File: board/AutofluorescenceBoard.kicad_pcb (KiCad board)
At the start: 2 copper layers, 57.2 x 45.7 mm, 41 parts, among them J1 2002411212, Q1 BSS138, U1 PAM2863ECR, U2 PAM2863ECR, U3 PAM2863ECR

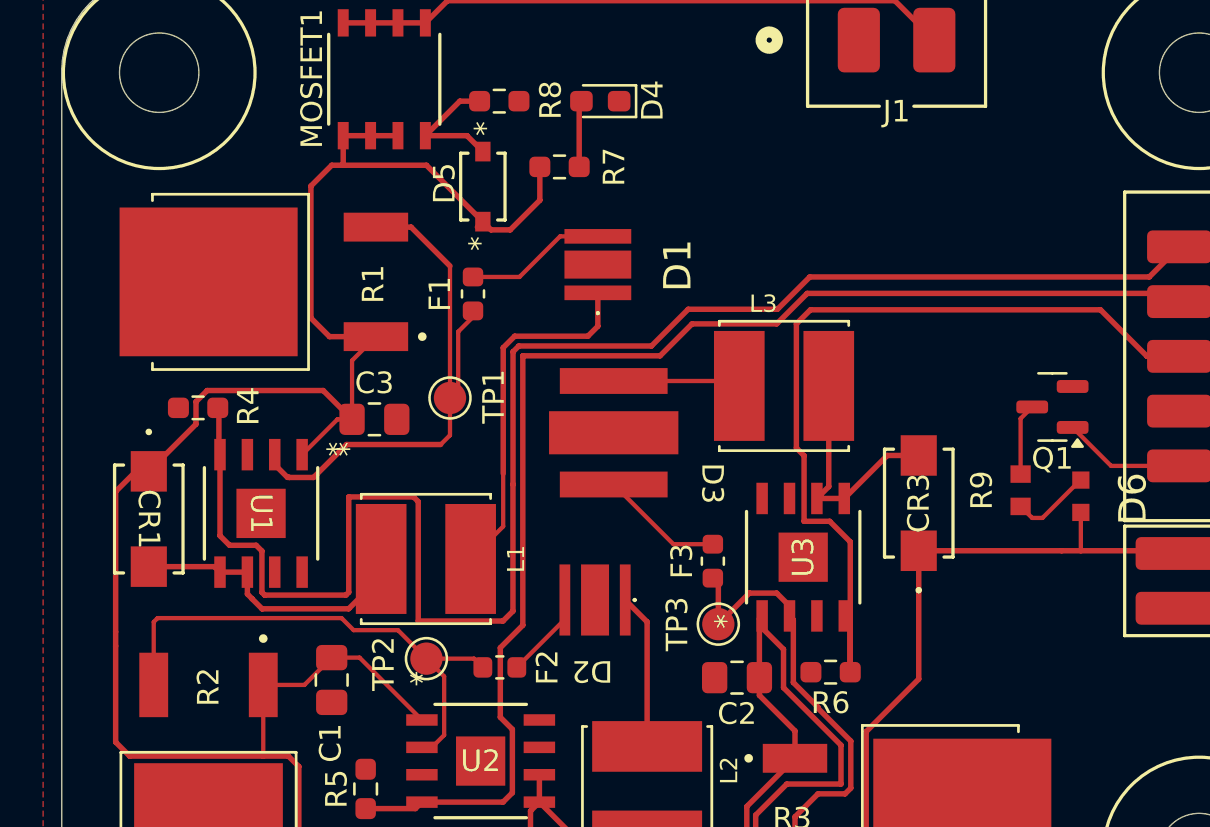
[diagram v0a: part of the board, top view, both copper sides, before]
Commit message: Silkscreens :)
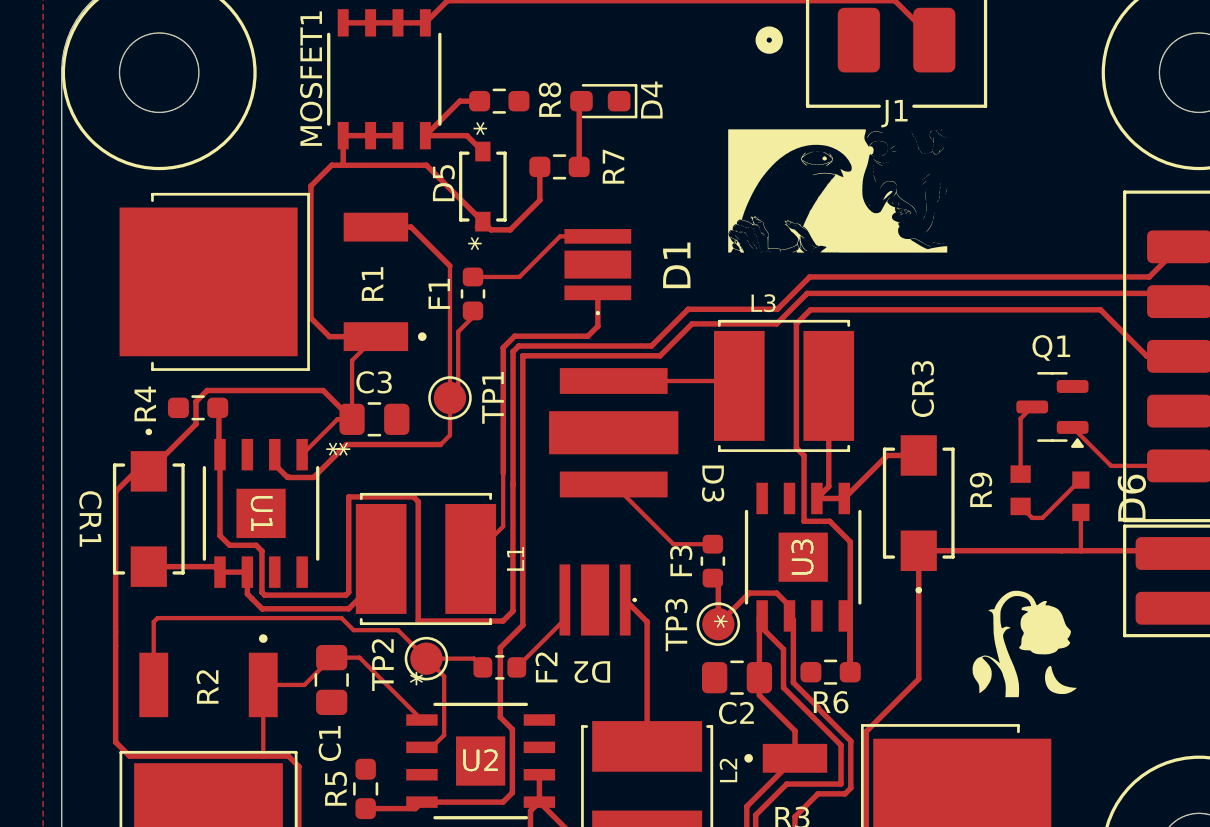
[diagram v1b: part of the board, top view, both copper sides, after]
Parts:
- added G***: LOGO, LOGO, F.Cu at (146.6, 137.6)
- added G***: LOGO, LOGO, F.Cu at (137.9, 116.7)

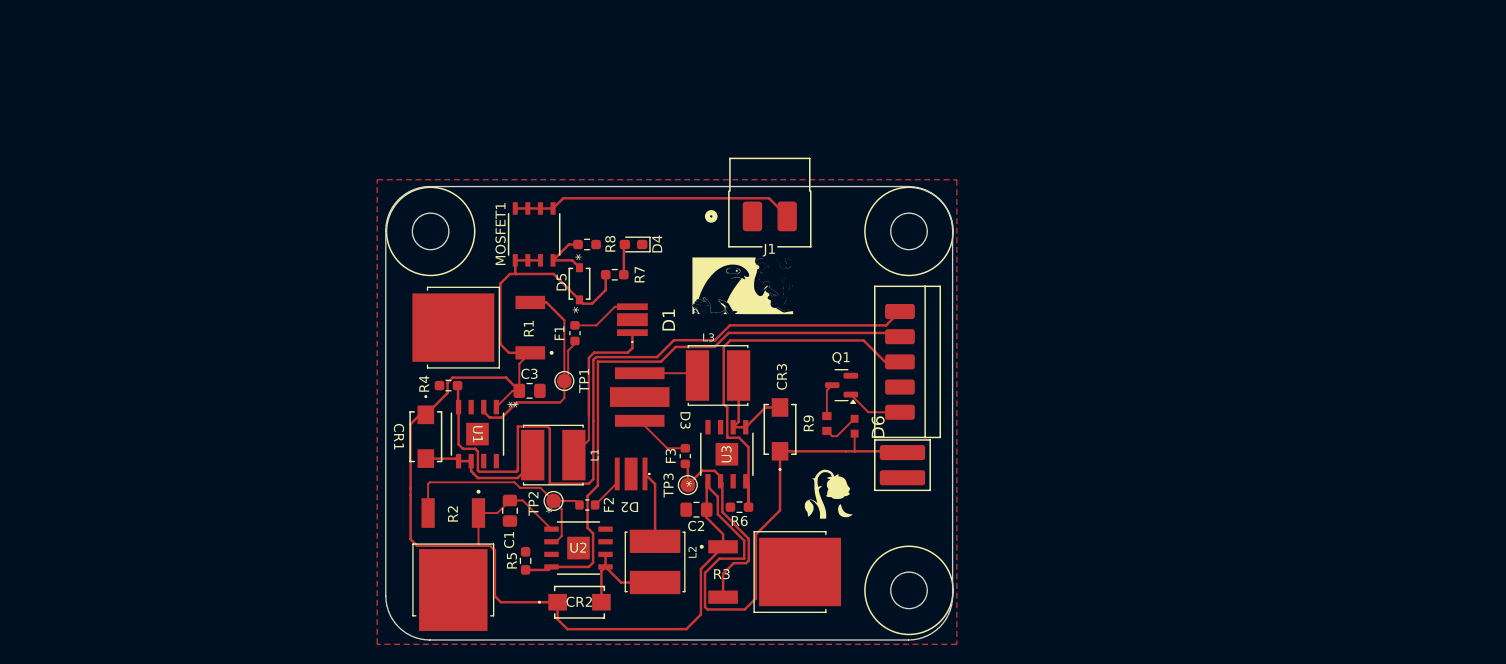
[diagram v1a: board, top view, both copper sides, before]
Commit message: Layout Changes from CDR
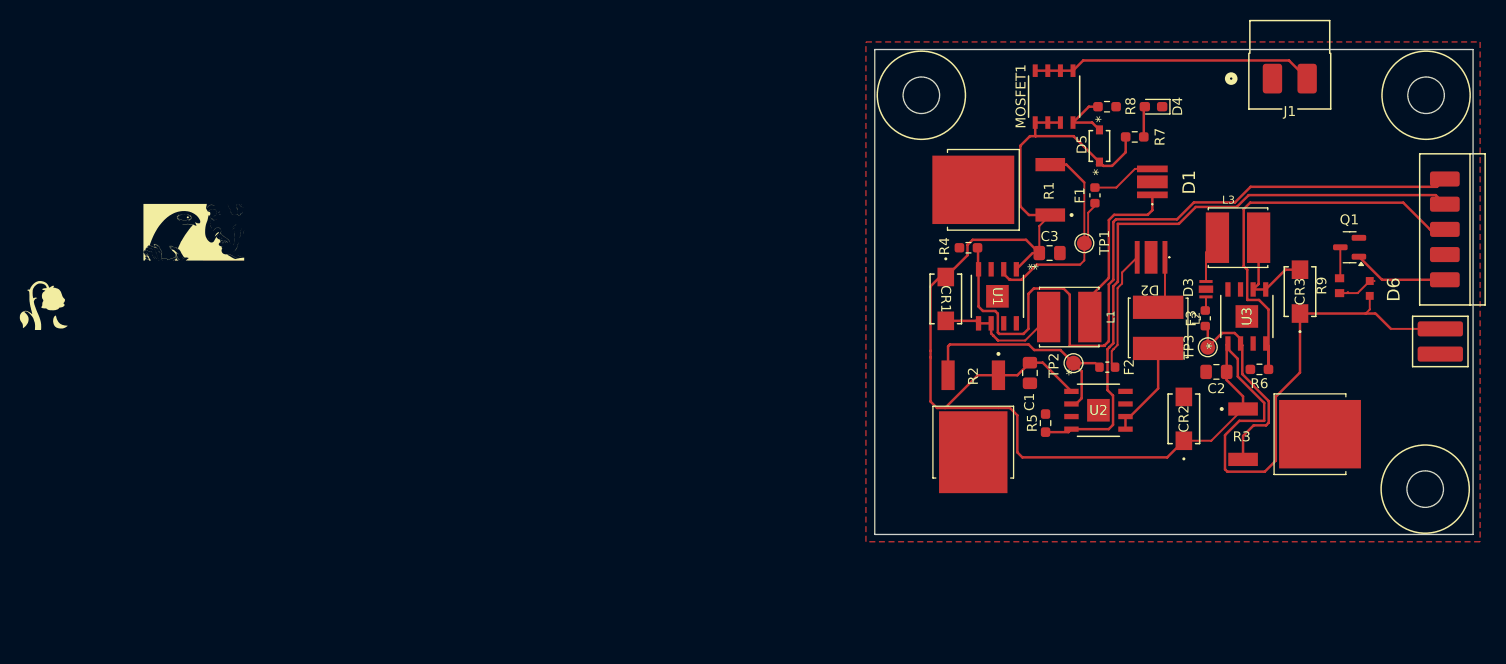
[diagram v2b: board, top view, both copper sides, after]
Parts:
- R3: value 0.3 -> 0.15
- R8: value 1K -> 10K
- moved G*** 81.4 mm to (67.5, 118.6)
- moved CR2 63.7 mm to (182.4, 130.1), turned to 90 degrees
- moved D3 61.7 mm to (185.7, 116.0)
- moved D2 56.8 mm to (180.5, 112.0)
- moved Conn1 56.5 mm to (208.7, 105.9)
- moved L2 55.9 mm to (179.8, 120.9)
- moved FanConn1 55.6 mm to (209.8, 121.0)
- moved G*** 55.6 mm to (82.6, 111.3)
- moved D1 54.2 mm to (179.2, 106.2)
- moved D4 54.2 mm to (179.4, 98.6)
- moved R1 54.2 mm to (163.8, 107.0)
- moved R4 54.2 mm to (160.7, 112.8)
- moved C1 54.2 mm to (166.9, 125.5)
- moved C3 54.2 mm to (168.9, 113.4)
- moved CR1 54.2 mm to (158.4, 118.0)
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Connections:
- J1 pad 2: Net-(J1-Pad2) -> unconnected-(J1-Pad2)
- MOSFET1 pad 5: Net-(J1-Pad2) -> GND
- MOSFET1 pad 6: Net-(J1-Pad2) -> GND
- MOSFET1 pad 7: Net-(J1-Pad2) -> GND
- MOSFET1 pad 8: Net-(J1-Pad2) -> GND
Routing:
- net Net-(J1-Pad2): track 28.6 -> 0.00 mm
- net (no net): track 0.00 -> 28.6 mm
- net Net-(D2-Pad2): track 4.06 -> 12.3 mm
- net Net-(D3-Pad2): track 5.74 -> 1.40 mm
- net White LED: track 5.69 -> 9.63 mm
- net ISET 490nm: track 39.5 -> 42.3 mm
- net ISET 405nm: track 59.9 -> 62.6 mm
- net Net-(D2-Pad1): track 7.21 -> 5.32 mm
- net ISET 365nm: track 77.1 -> 78.4 mm
- net +12V: track 179.2 -> 177.9 mm
- net Net-(D3-Pad1): track 6.24 -> 5.22 mm
- net Net-(CR2-Pad2): track 10.6 -> 9.77 mm
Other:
- board size 57.2 x 45.7 mm -> 60.3 x 48.9 mm
- board text removed: "increase width by .01 increase length by .03"
